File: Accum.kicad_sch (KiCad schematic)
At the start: 0 parts

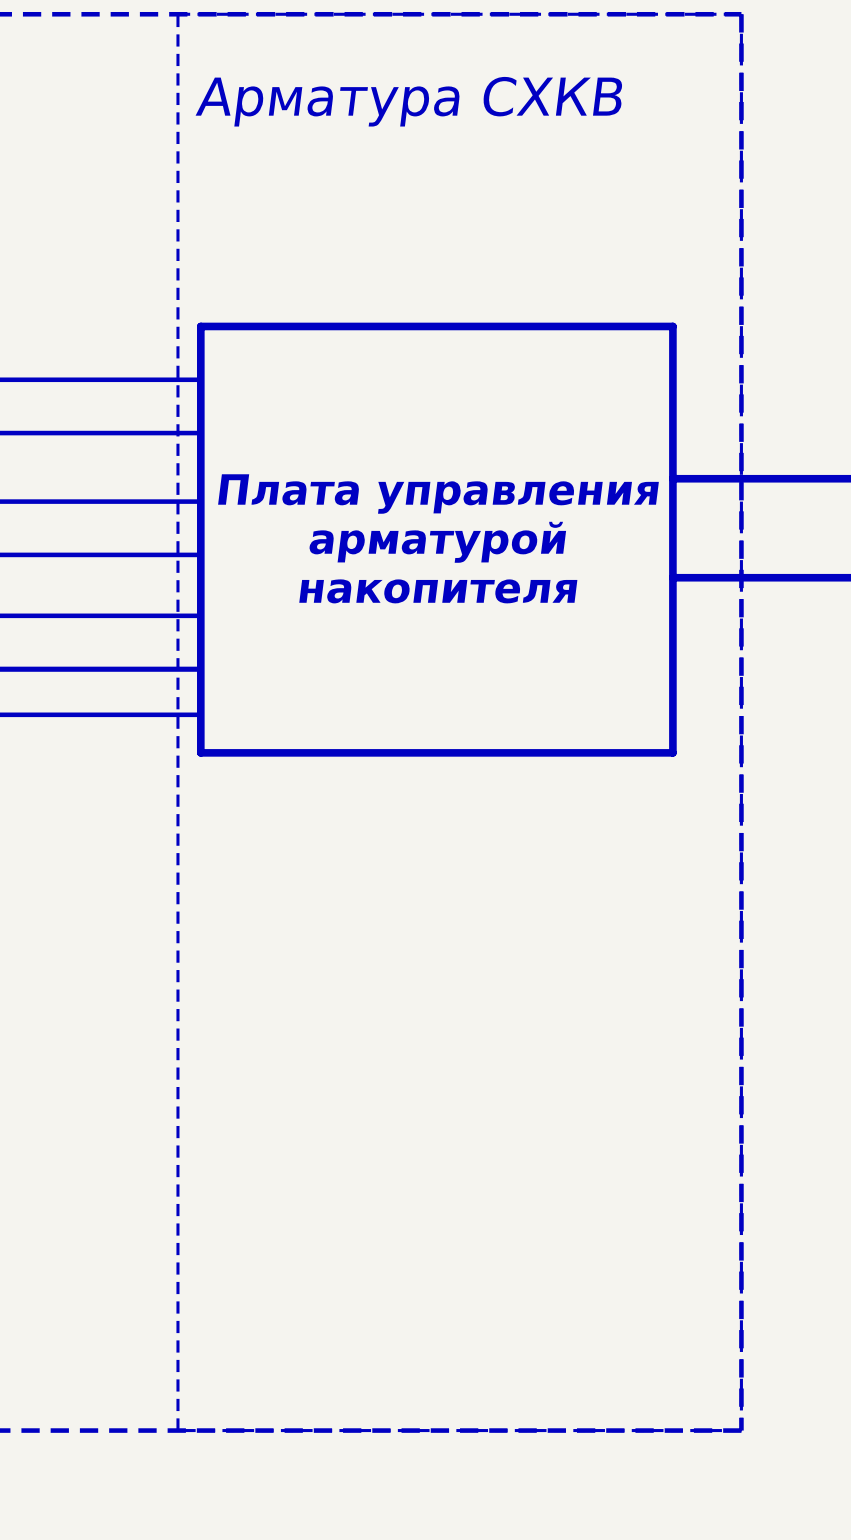
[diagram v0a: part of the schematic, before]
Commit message: version for piter
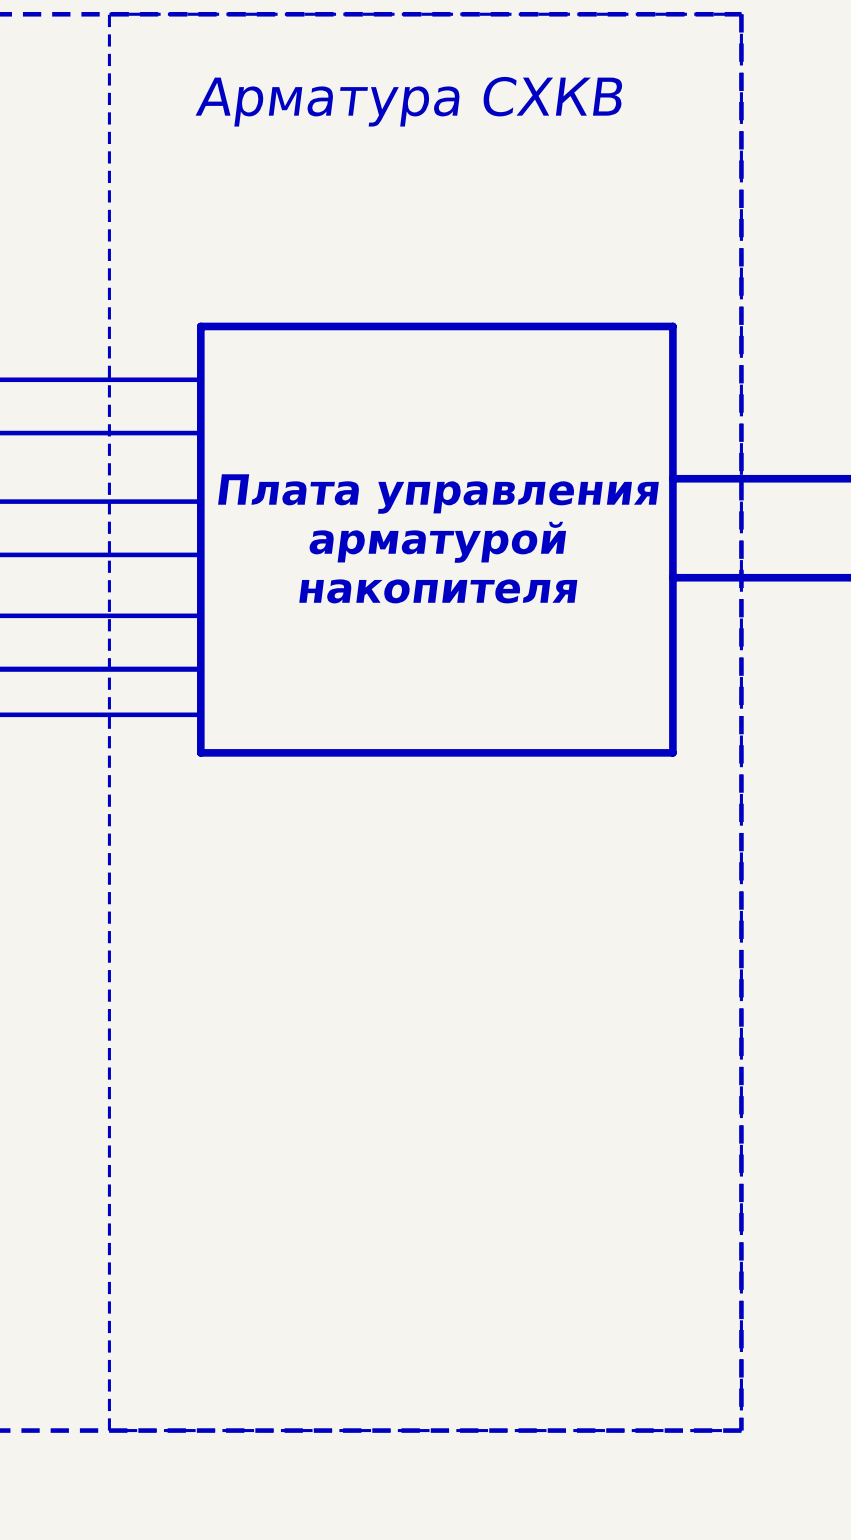
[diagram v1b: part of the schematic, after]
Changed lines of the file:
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@@
 	)
 	(rectangle
-		(start 396.24 88.9)
+		(start 384.81 88.9)
 		(end 490.22 325.12)
 		(stroke
